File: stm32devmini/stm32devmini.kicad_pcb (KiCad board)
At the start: 2 copper layers, 52.1 x 20.3 mm, 30 parts, among them J1 USB_B_Micro, SW1 SW_Push, U1 AMS1117-3.3, U2 STM32F103C8Tx, Y1 8M, Y2 32.768k

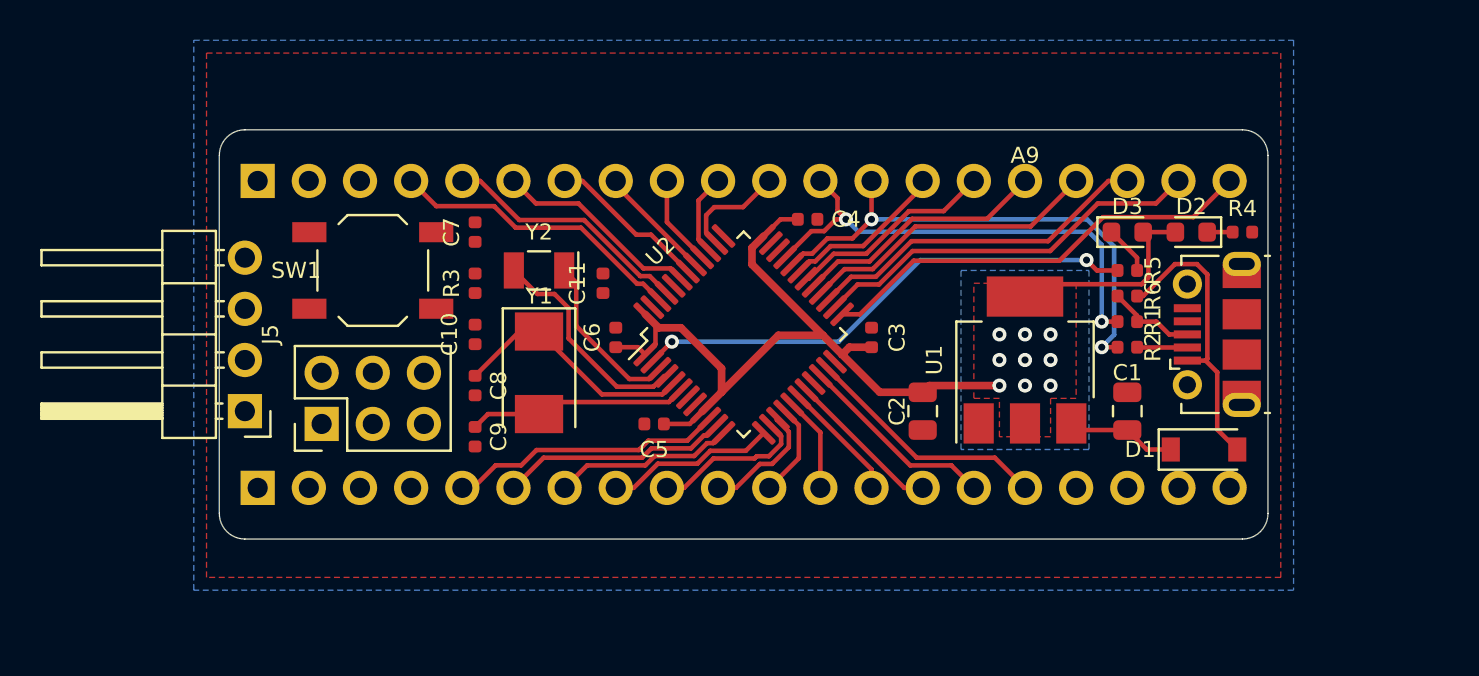
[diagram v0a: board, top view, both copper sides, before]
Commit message: Hmmmm
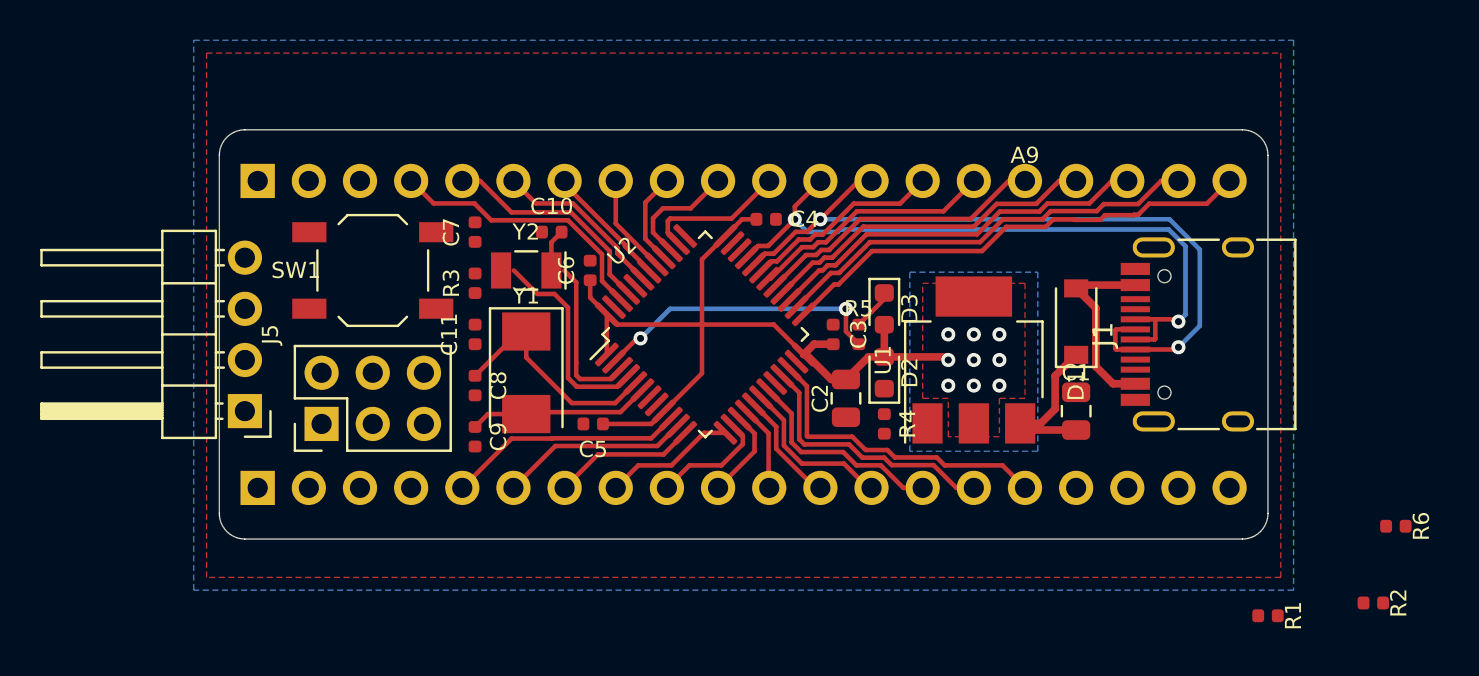
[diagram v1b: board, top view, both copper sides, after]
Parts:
- J1: value USB_B_Micro -> USB_C_Receptacle_USB2.0; footprint Connector_USB:USB_Micro-B_Molex-105017-0001 -> Connector_USB:USB_C_Receptacle_HRO_TYPE-C-31-M-12
- moved R4 20.2 mm to (184.8, 106.0), turned to 270 degrees
- moved R2 17.6 mm to (209.1, 114.9)
- moved R6 17.6 mm to (210.2, 111.1)
- moved D2 16.8 mm to (184.8, 103.5), turned to 90 degrees
- moved R1 16.2 mm to (203.8, 115.6)
- moved R5 13.7 mm to (183.5, 101.6), turned to 270 degrees
- moved D3 12.7 mm to (184.8, 100.3), turned to 270 degrees
- moved D1 8.98 mm to (194.3, 101.0), turned to 90 degrees
- moved C11 6.84 mm to (164.5, 101.6)
- moved C10 6.35 mm to (168.3, 96.5), turned to 180 degrees
- moved C2 3.86 mm to (182.9, 104.8)
- moved C6 3.56 mm to (170.2, 98.4)
- moved C5 3.02 mm to (170.3, 106.0)
- moved U1 2.54 mm to (189.2, 102.9)
- moved C1 2.54 mm to (194.3, 105.4)
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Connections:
- J2 pad 1: Net-(J2-Pad1) -> VBUS
- J2 pad 17: Net-(J2-Pad17) -> RST
- J2 pad 18: Net-(J2-Pad18) -> +3V3
- J2 pad 19: Net-(J2-Pad19) -> GND
- J2 pad 20: Net-(J2-Pad20) -> GND
- R1 pad 1: Net-(J1-Pad3) -> Net-(R1-Pad1)
- R1 pad 2: A12 -> Net-(R1-Pad2)
- R2 pad 1: Net-(J1-Pad2) -> Net-(R2-Pad1)
- R2 pad 2: A11 -> Net-(R2-Pad2)
- R6 pad 2: Net-(J1-Pad3) -> Net-(R1-Pad1)
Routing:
- net A11: track 25.4 -> 37.4 mm
- net C13: track 25.4 -> 14.6 mm
- net A12: track 24.1 -> 33.7 mm
- net +3V3: track 50.7 -> 41.3 mm
- net Net-(D1-Pad2): track 14.6 -> 9.61 mm
- net Net-(J1-Pad3): track 4.43 -> 0.00 mm
- net B11: track 12.2 -> 15.6 mm
- net B10: track 9.91 -> 13.2 mm
- net B1: track 7.78 -> 10.5 mm
- net VBUS: track 5.48 -> 8.07 mm
- net Net-(J1-Pad2): track 2.50 -> 0.00 mm
- net B0: track 5.98 -> 8.09 mm
- net B12: track 22.0 -> 23.9 mm
- net A8: track 12.7 -> 14.6 mm
- net A2: track 9.02 -> 7.12 mm
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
